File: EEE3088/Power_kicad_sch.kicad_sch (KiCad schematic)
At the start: 28 parts, among them U1 TP4056, U2 HT7533-1

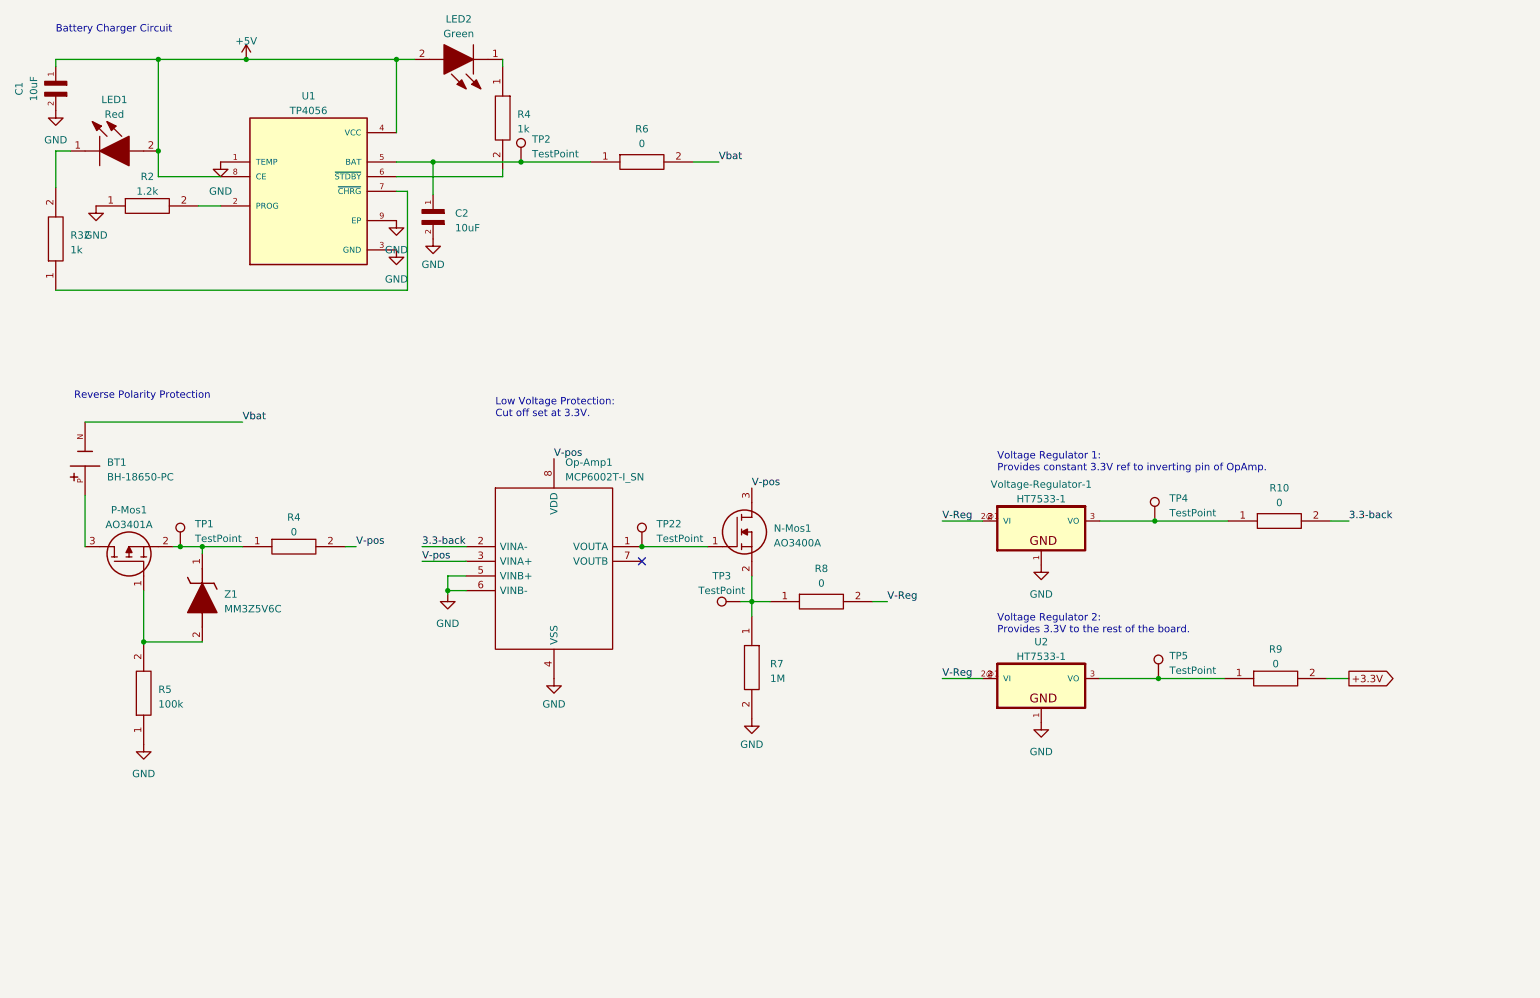
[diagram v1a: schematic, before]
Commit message: H_1
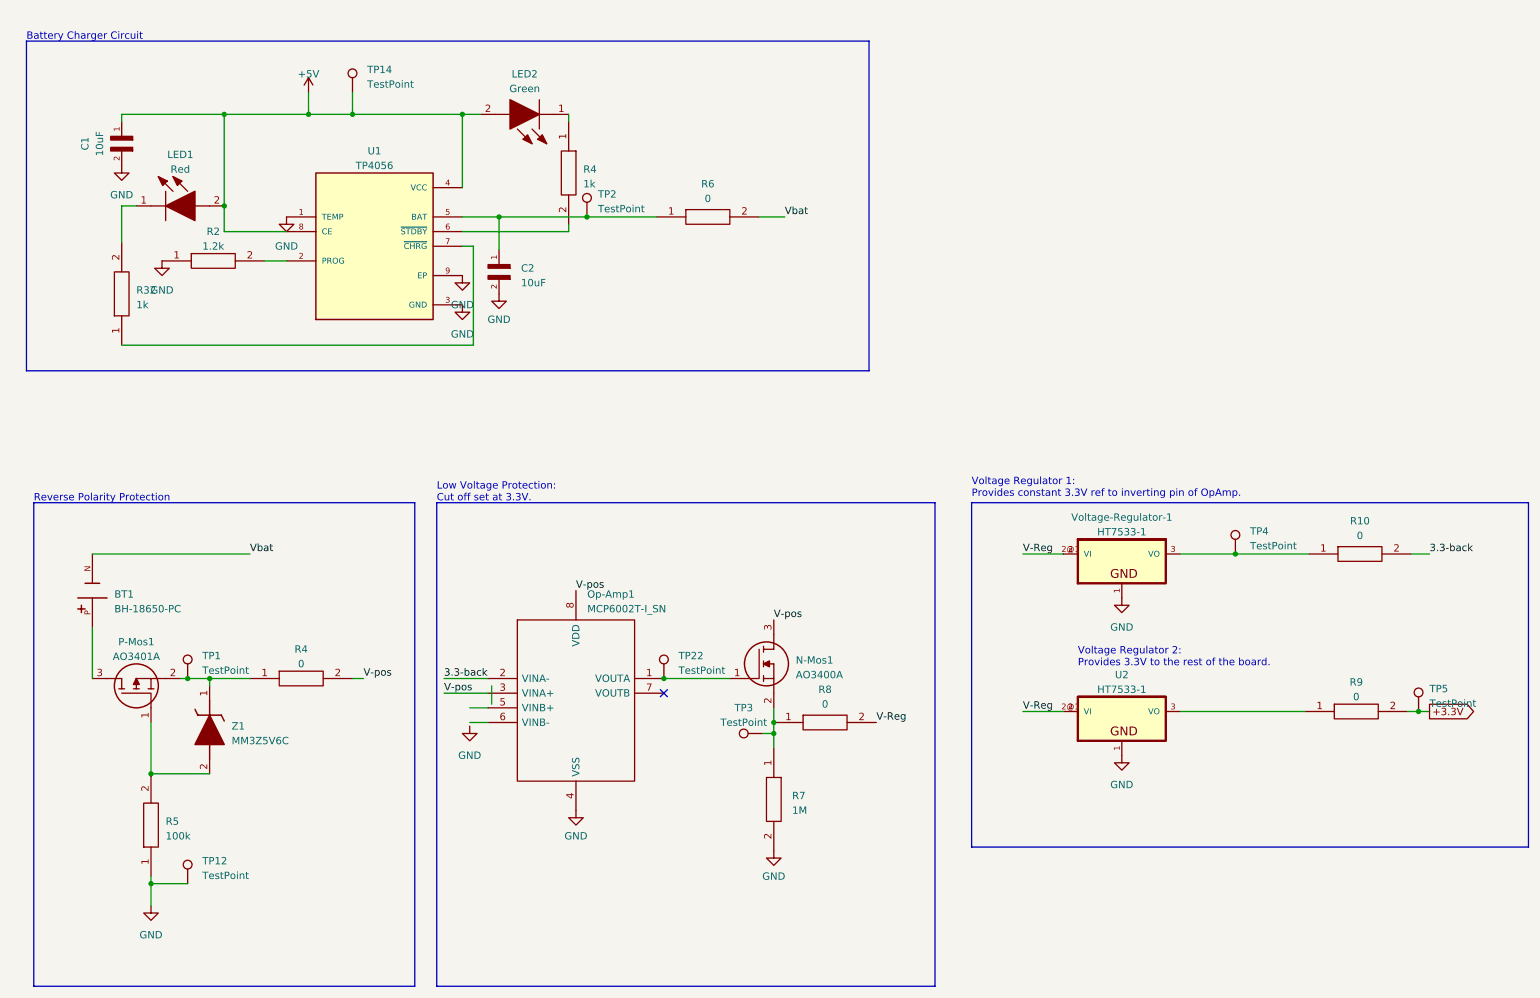
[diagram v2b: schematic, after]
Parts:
- added TP12, TP14: TestPoint, TestPoint:TestPoint_Pad_2.0x2.0mm, symbol Connector:TestPoint
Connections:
- net +3.3V: now also TP5.1
- net +5V: now also TP14.1
- net GND: now also TP12.1; no longer Op-Amp1.5 (VINB+), Op-Amp1.6 (VINB-)
- net at R9.1, U2.3 (VO): no longer TP5.1
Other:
- moved on the sheet: BT1, C1, C2, LED1, LED2, N-Mos1, Op-Amp1, P-Mos1, R10, R2, R32, R4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

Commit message: Schematic updates
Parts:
- BT1: JLC Part Number (none) -> DNP; Manufacturer_Part_Number - -> DNP; Price 0.00 -> 0
- C1, C2: JLC Part Number C19702 -> C15850; Manufacturer_Part_Number CL10A106KP8NNNC -> CL21A106KAYNNNE; Price 0.0066 -> 0.0131
- N-Mos1: Price 0.0864 -> 0.0787
- Op-Amp1: Price 0.282 -> 0.2660
- P-Mos1: Price 0.0797 -> 0.0765
- R10, R4, R6, R8, R9: JLC Part Number C17168 -> C17477; Manufacturer_Part_Number 0402WGF0000TCE -> 0805W8F0000T5E; Price 0.0035 -> 0.0022
- R2: JLC Part Number C22765 -> C17379; Manufacturer_Part_Number 0603WAF1201T5E -> 0805W8F1201T5E; Price 0.001 -> 0.0018
- R32, R4: JLC Part Number C21190 -> C17513; Manufacturer_Part_Number 0603WAF1001T5E -> 0805W8F1001T5E; Price 0.0006 -> 0.0021
- R5: JLC Part Number C17900 -> C149504; Manufacturer_Part_Number 1206W4F1003T5E -> 0805W8F1003T5E; Price 0.0032 -> 0.0017
- TP1, TP12, TP14, TP2, TP3, TP4, TP5: JLC Part Number (none) -> DNP; Manufacturer_Part_Number 0 -> DNP
- TP22: Extended (none) -> 0; JLC Part Number (none) -> DNP; Manufacturer_Part_Number (none) -> DNP; Price (none) -> 0
- U1: Price 0.2064 -> 0.2121
- U2, Voltage-Regulator-1: Price 0.1315 -> 0.1279
- Z1: Manufacturer_Part_Number MM3Z5V6C -> MM3Z5V6; Price 0.0184 -> 0.0182

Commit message: Schematic + PCB Update
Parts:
- C1, C2: footprint CL10A106KP8NNNC:CAPC1608X90N -> Capacitor_SMD:C_0805_2012Metric
- R10, R4, R6, R8, R9: footprint Resistor_SMD:R_0402_1005Metric -> Resistor_SMD:R_0805_2012Metric
- R2: footprint My1.2k:RESC1608X55N -> Resistor_SMD:R_0805_2012Metric
- R32, R4: footprint RESC1608X55N -> Resistor_SMD:R_0805_2012Metric
- R5: footprint My100k:RESC3116X65N -> Resistor_SMD:R_0805_2012Metric
- R7: footprint My1M:RESC2013X65N -> Resistor_SMD:R_0805_2012Metric
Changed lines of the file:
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@@
       (effects (font (size 1.27 1.27)) (justify left))
     )
-    (property "Footprint" "My1M:RESC2013X65N" (at 148.59 158.115 0)
+    (property "Footprint" "Resistor_SMD:R_0805_2012Metric" (at 148.59 158.115 0)
       (effects (font (size 1.27 1.27)) (justify left) hide)
     )
@@
       (effects (font (size 1.27 1.27)) (justify right))
     )
-    (property "Footprint" "My100k:RESC3116X65N" (at 38.1 152.4 0)
+    (property "Footprint" "Resistor_SMD:R_0805_2012Metric" (at 38.1 152.4 0)
       (effects (font (size 1.27 1.27)) (justify left) hide)
     )
@@
       (effects (font (size 1.27 1.27)) (justify left))
     )
-    (property "Footprint" "RESC1608X55N" (at 113.03 49.53 0)
+    (property "Footprint" "Resistor_SMD:R_0805_2012Metric" (at 113.03 49.53 0)
       (effects (font (size 1.27 1.27)) (justify left) hide)
     )
@@
       (effects (font (size 1.27 1.27)) (justify left) hide)
     )
-    (property "Description" "1k Res 0805" (at 107.95 49.53 0)
+    (property "Description" "1k Resistor 0805" (at 107.95 49.53 0)
       (effects (font (size 1.27 1.27)) (justify left) hide)
     )
@@
       (effects (font (size 1.27 1.27)))
     )
-    (property "Footprint" "Resistor_SMD:R_0402_1005Metric" (at 253.365 136.525 0)
+    (property "Footprint" "Resistor_SMD:R_0805_2012Metric" (at 253.365 136.525 0)
       (effects (font (size 1.27 1.27)) (justify left) hide)
     )
@@
       (effects (font (size 1.27 1.27)) (justify left) hide)
     )
-    (property "Description" "0 Res 0805" (at 253.365 141.605 0)
+    (property "Description" "0 Resistor 0805" (at 253.365 141.605 0)
       (effects (font (size 1.27 1.27)) (justify left) hide)
     )
@@
       (effects (font (size 1.27 1.27)))
     )
-    (property "Footprint" "CL10A106KP8NNNC:CAPC1608X90N" (at 34.29 40.64 0)
+    (property "Footprint" "Capacitor_SMD:C_0805_2012Metric" (at 34.29 40.64 0)
       (effects (font (size 1.27 1.27)) (justify bottom) hide)
     )
@@
       (effects (font (size 1.27 1.27)))
     )
-    (property "Footprint" "Resistor_SMD:R_0402_1005Metric" (at 254 109.22 0)
+    (property "Footprint" "Resistor_SMD:R_0805_2012Metric" (at 254 109.22 0)
       (effects (font (size 1.27 1.27)) (justify left) hide)
     )
@@
       (effects (font (size 1.27 1.27)) (justify left) hide)
     )
-    (property "Description" "0 Res 0805" (at 254 114.3 0)
+    (property "Description" "0 Resistor 0805" (at 254 114.3 0)
       (effects (font (size 1.27 1.27)) (justify left) hide)
     )
@@
       (effects (font (size 1.27 1.27)))
     )
-    (property "Footprint" "Resistor_SMD:R_0402_1005Metric" (at 161.29 138.43 0)
+    (property "Footprint" "Resistor_SMD:R_0805_2012Metric" (at 161.29 138.43 0)
       (effects (font (size 1.27 1.27)) (justify left) hide)
     )
@@
       (effects (font (size 1.27 1.27)) (justify left) hide)
     )
-    (property "Description" "0 Res 0805" (at 161.29 143.51 0)
+    (property "Description" "0 Resistor 0805" (at 161.29 143.51 0)
       (effects (font (size 1.27 1.27)) (justify left) hide)
     )
@@
       (effects (font (size 1.27 1.27)) (justify right))
     )
-    (property "Footprint" "CL10A106KP8NNNC:CAPC1608X90N" (at 99.695 62.865 0)
+    (property "Footprint" "Capacitor_SMD:C_0805_2012Metric" (at 99.695 62.865 0)
       (effects (font (size 1.27 1.27)) (justify bottom) hide)
     )
@@
       (effects (font (size 1.27 1.27)))
     )
-    (property "Footprint" "Resistor_SMD:R_0402_1005Metric" (at 140.97 50.8 0)
+    (property "Footprint" "Resistor_SMD:R_0805_2012Metric" (at 140.97 50.8 0)
       (effects (font (size 1.27 1.27)) (justify left) hide)
     )
@@
       (effects (font (size 1.27 1.27)) (justify left) hide)
     )
-    (property "Description" "0 Res 0805" (at 140.97 55.88 0)
+    (property "Description" "0 Resistor 0805" (at 140.97 55.88 0)
       (effects (font (size 1.27 1.27)) (justify left) hide)
     )
@@
       (effects (font (size 1.27 1.27)))
     )
-    (property "Footprint" "Resistor_SMD:R_0402_1005Metric" (at 70.485 130.81 0)
+    (property "Footprint" "Resistor_SMD:R_0805_2012Metric" (at 70.485 130.81 0)
       (effects (font (size 1.27 1.27)) (justify left) hide)
     )
@@
       (effects (font (size 1.27 1.27)) (justify left) hide)
     )
-    (property "Description" "0 Res 0805" (at 70.485 135.89 0)
+    (property "Description" "0 Resistor 0805" (at 70.485 135.89 0)
       (effects (font (size 1.27 1.27)) (justify left) hide)
     )
@@
       (effects (font (size 1.27 1.27)) (justify right))
     )
-    (property "Footprint" "RESC1608X55N" (at 33.02 60.325 0)
+    (property "Footprint" "Resistor_SMD:R_0805_2012Metric" (at 33.02 60.325 0)
       (effects (font (size 1.27 1.27)) (justify left) hide)
     )
@@
       (effects (font (size 1.27 1.27)) (justify left) hide)
     )
-    (property "Description" "1k Res 0805" (at 38.1 60.325 0)
+    (property "Description" "1k Resistor 0805" (at 38.1 60.325 0)
       (effects (font (size 1.27 1.27)) (justify left) hide)
     )
@@
       (effects (font (size 1.27 1.27)))
     )
-    (property "Footprint" "My1.2k:RESC1608X55N" (at 43.815 67.945 0)
-      (effects (font (size 1.27 1.27)) (justify left) hide)
-    )
+    (property "Footprint" "Resistor_SMD:R_0805_2012Metric" (at 43.815 67.945 0)
+      (effects (font (size 1.27 1.27)) (justify left) hide)
+    )
